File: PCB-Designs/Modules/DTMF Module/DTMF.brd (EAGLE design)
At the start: 18 parts, among them IC1 CM8870CP

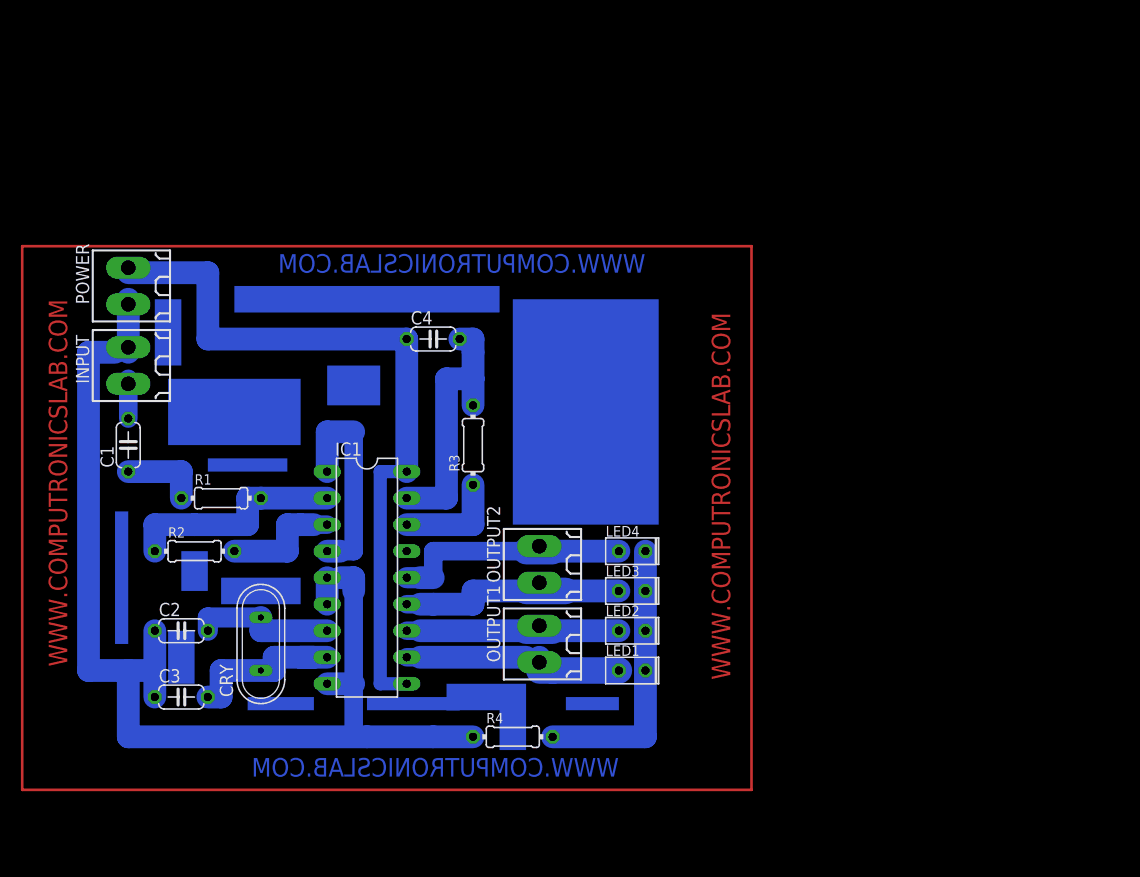
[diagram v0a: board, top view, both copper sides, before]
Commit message: change
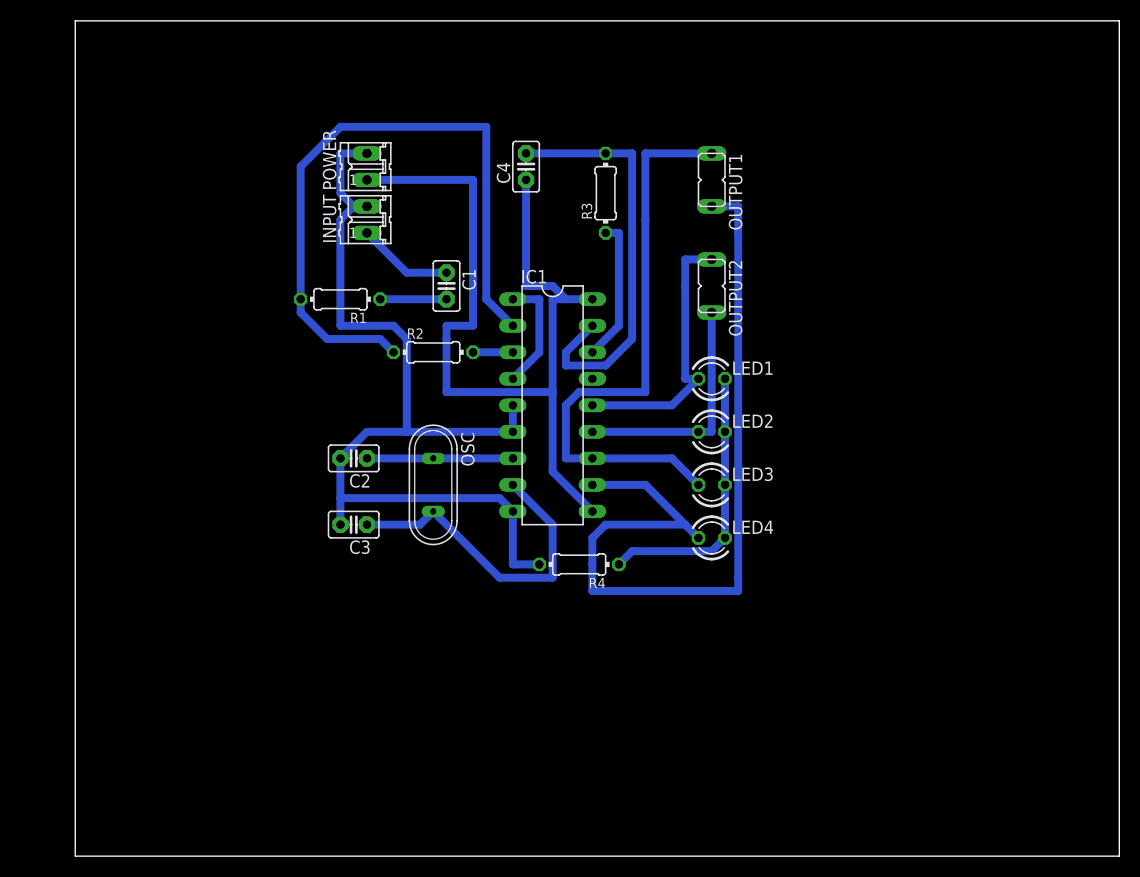
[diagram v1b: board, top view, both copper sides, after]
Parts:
- removed CRY: 3.57, special:QS
- added OSC: 3.57, special:QS
- C1: value 0.47UF -> 0.47uf; device resistor:C050-024X044 -> capacitor-wima:C2.5-2
- C2, C3, C4: device resistor:C050-024X044 -> capacitor-wima:C2.5-2
- INPUT, POWER: device con-weidmueller-sl35:180-2 -> con-amp-quick:02P
- LED1, LED2, LED3, LED4: value (none) -> 3mm; device led:LED2X5 -> led:LED3MM
- OUTPUT1, OUTPUT2: device con-weidmueller-sl35:180-2 -> jumper:JP1
- R4: value 330 -> 330E
- moved OUTPUT1 47.4 mm to (61.0, 64.8), turned to 180 degrees
- moved C1 34.1 mm to (35.6, 54.6), turned to 270 degrees
- moved OUTPUT2 31.4 mm to (61.0, 54.6), turned to 180 degrees
- moved R2 29.8 mm to (34.3, 48.3)
- moved LED1 29.0 mm to (61.0, 45.7)
- moved R3 27.3 mm to (50.8, 63.5)
- moved INPUT 26.8 mm to (27.9, 61.0)
- moved POWER 25.6 mm to (27.9, 66.0)
- moved IC1 24.3 mm to (45.7, 43.2)
- moved C2 23.3 mm to (26.7, 38.1), turned to 180 degrees
- moved C3 23.3 mm to (26.7, 31.8), turned to 180 degrees
- moved R1 22.2 mm to (25.4, 53.3), turned to 180 degrees
- moved LED2 20.5 mm to (61.0, 40.6)
- moved C4 18.8 mm to (43.2, 66.0), turned to 90 degrees
- moved R4 17.7 mm to (48.3, 27.9), turned to 180 degrees
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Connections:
- net S$1 renamed N$12
- net S$8 renamed N$3
- removed net N$13 (its old number): C1.1, R1.1
- removed net N$17 (its old number): POWER.1
- removed net N$21: C2.1, C3.1, IC1.9, R4.1
- removed net N$22: IC1.5, IC1.6
- removed net N$23: IC1.14, LED4.A
- removed net N$24 (its old number): IC1.13, LED3.A
- removed net N$26: IC1.10, IC1.18
- removed net S$10: IC1.11
- removed net S$11: IC1.12, LED2.A
- removed net S$17: LED1.A
- removed net S$18: LED1.K, LED2.K, LED3.K, LED4.K, R4.2
- removed net S$2: C1.2
- removed net S$4: C2.2
- removed net S$5: C3.2, IC1.8
- new net N$1: C2.2, C3.2, IC1.5, IC1.6, IC1.9, INPUT.2, POWER.2, R4.2
- new net N$10: C4.1, IC1.10, IC1.18, POWER.1
- new net N$11: C1.1, INPUT.1
- new net N$14: C2.1, IC1.7, OSC.1
- new net N$15: C3.1, IC1.8, OSC.2
- new net N$2: C1.2, R1.1
- new net N$5: IC1.11, LED4.A, OUTPUT1.2
- new net N$6: IC1.12, LED3.A, OUTPUT1.1
- new net N$7: IC1.13, LED2.A, OUTPUT2.2
- new net N$8: IC1.14, LED1.A, OUTPUT2.1
- net N$4: now also LED1.K, LED2.K, LED3.K, LED4.K, R4.1; no longer POWER.2
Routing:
- net S$3: track 243.8 -> 0.00 mm
- net N$21: track 106.7 -> 0.00 mm
- net N$1: track 0.00 -> 89.5 mm
- net N$10: track 0.00 -> 83.4 mm
- net N$5: track 0.00 -> 80.1 mm
- net N$26: track 71.1 -> 0.00 mm
- net N$6: track 0.00 -> 56.2 mm
- net N$12: track 21.6 -> 63.9 mm
- net N$15: track 0.00 -> 31.4 mm
- net S$18: track 26.7 -> 0.00 mm
- net N$4: track 0.00 -> 26.5 mm
- net N$8: track 0.00 -> 26.5 mm
- net N$24 (its old number): track 24.1 -> 0.00 mm
- net N$23: track 24.1 -> 0.00 mm
- net N$7: track 0.00 -> 22.9 mm
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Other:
- board outline added: 100 x 80 mm
- board text removed: "WWW.COMPUTRONICSLAB.COM"
